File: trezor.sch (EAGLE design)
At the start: 35 parts, among them IC1 MCP1703CB, Q2 16MHz, U1 ATSHA204-TSU, U2 USB, U3 DISPLAY, X3 SSW-103-02-S-D

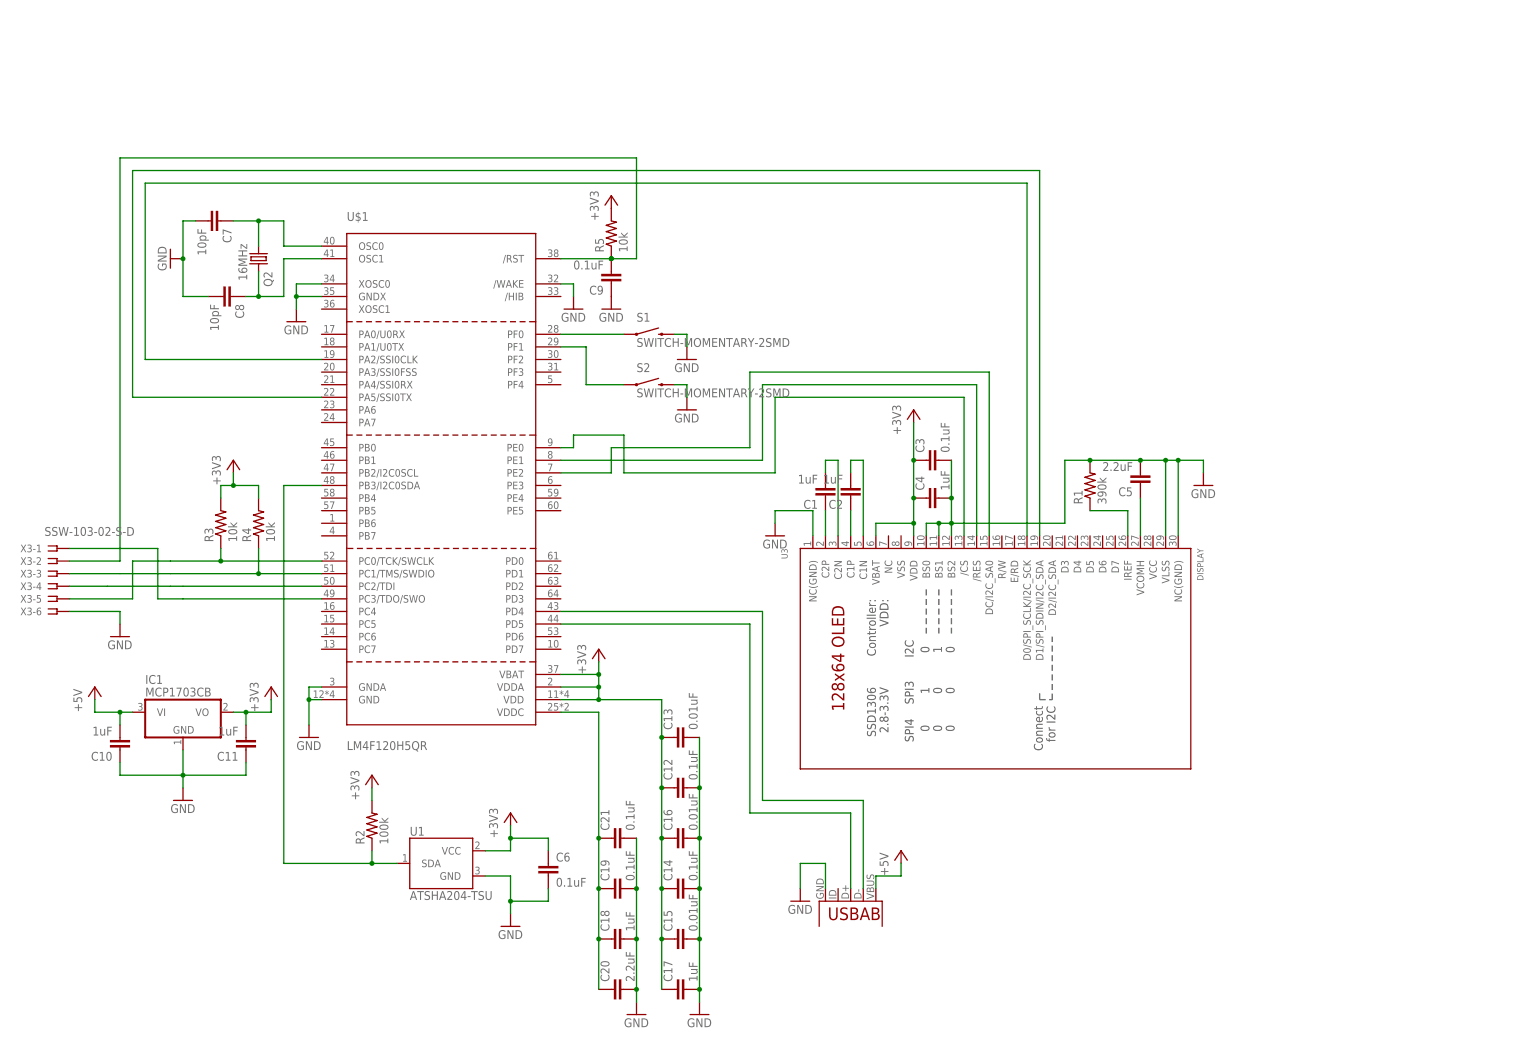
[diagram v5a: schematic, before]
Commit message: rework to STM32 (WIP)
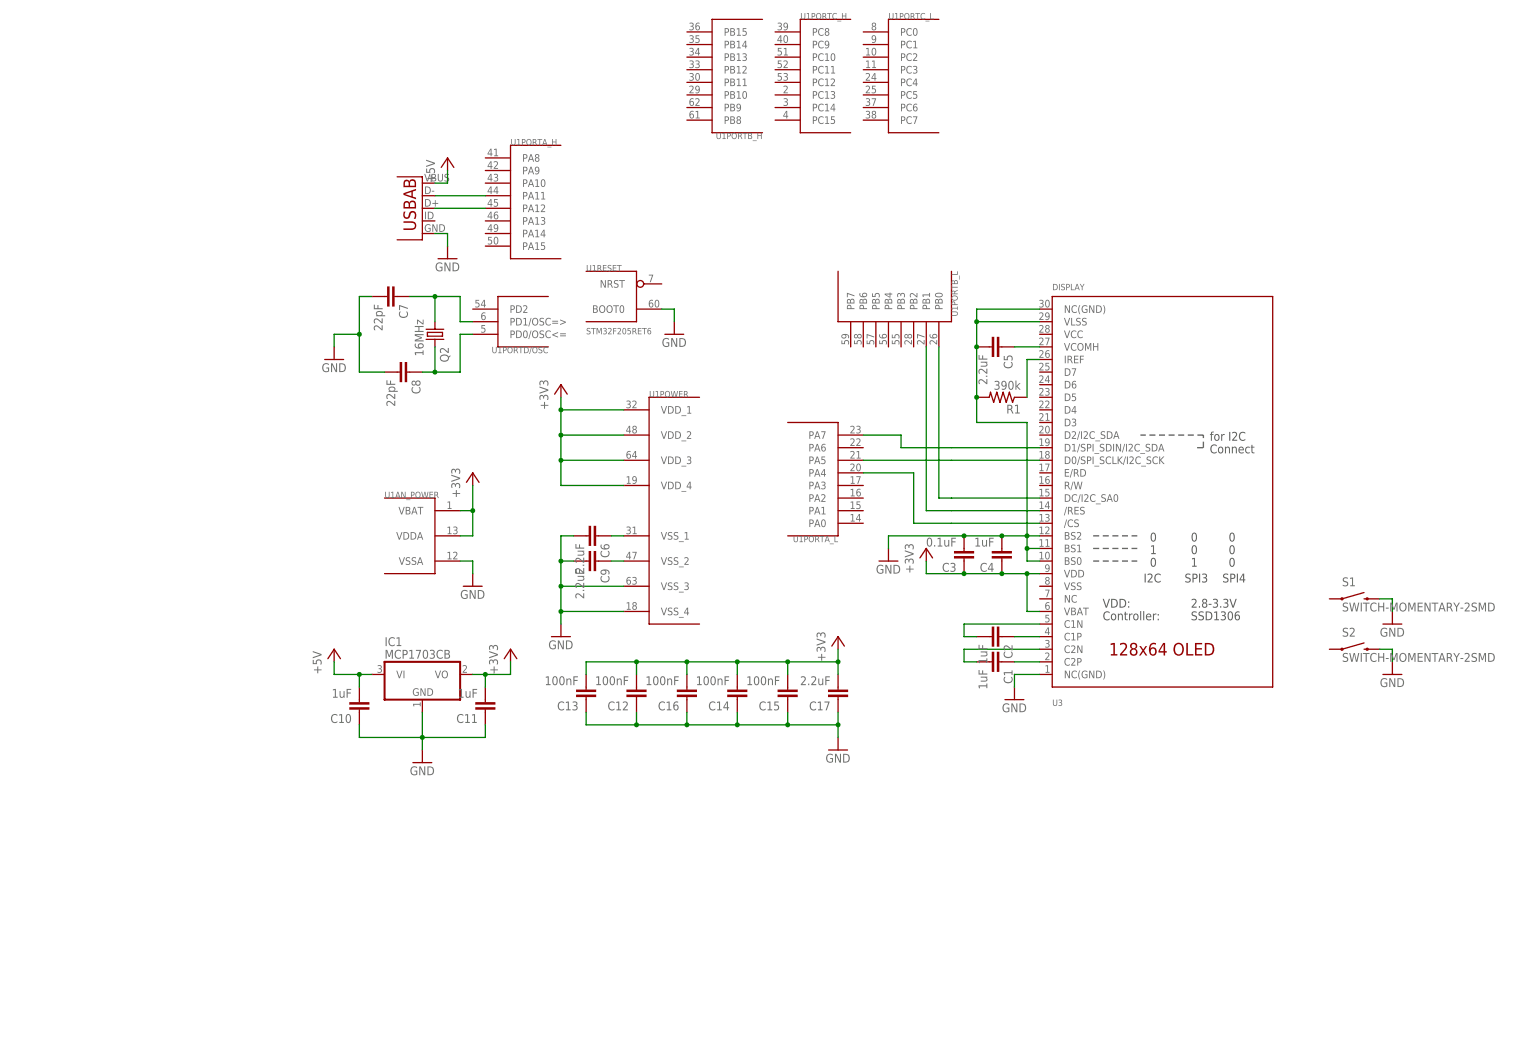
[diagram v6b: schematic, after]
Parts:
- removed C18: 1uF, SparkFun-Passives:CAP0402-CAP
- removed C19, C21: 0.1uF, SparkFun-Passives:CAP0402-CAP
- removed C20: 2.2uF, SparkFun-Passives:CAP0805
- removed R2: 100k, SparkFun-Passives:RESISTOR0402-RES
- removed R3, R4, R5: 10k, SparkFun-Passives:RESISTOR0402-RES
- removed U$1: LM4F120H5QR, stellaris:LM4F120H5QR
- removed X3: SSW-103-02-S-D, con-samtec:SSW-103-02-S-D
- C1, C10, C11, C2, C3, C4, C5: device SparkFun-Passives:CAP0402-CAP -> SparkFun-Passives:CAP0603-CAP
- C12, C14: value 0.1uF -> 100nF; device SparkFun-Passives:CAP0402-CAP -> SparkFun-Passives:CAP0603-CAP
- C13, C15, C16: value 0.01uF -> 100nF; device SparkFun-Passives:CAP0402-CAP -> SparkFun-Passives:CAP0603-CAP
- C17: value 1uF -> 2.2uF; device SparkFun-Passives:CAP0402-CAP -> SparkFun-Passives:CAP0603-CAP
- C6, C9: value 0.1uF -> 2.2uF; device SparkFun-Passives:CAP0402-CAP -> SparkFun-Passives:CAP0603-CAP
- C7, C8: value 10pF -> 22pF; device SparkFun-Passives:CAP0402-CAP -> SparkFun-Passives:CAP0603-CAP
- R1: device SparkFun-Passives:RESISTOR0402-RES -> SparkFun-Passives:RESISTOR0603-RES
- U1: value ATSHA204-TSU -> STM32F205RET6; device SparkFun-DigitalIC:ATSHA204-TSU -> stm32:STM32F10XRXT6
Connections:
- removed net N$15: S1.1, U$1.PF0
- removed net N$17: R3.1, U$1.PC0/TCK/SWCLK, X3-5.1
- removed net N$19: U$1.PC2/TDI, X3-4.1
- removed net N$20: U$1.PC3/TDO/SWO, X3-1.1
- removed net N$21: C9.2, R5.1, U$1./RST, X3-2.1
- removed net N$23: C18.1, C19.1, C20.1, C21.1, U$1.VDDC
- removed net SDA: R2.1, U$1.PB3/I2C0SDA, U1.SDA
- removed net USB_D_N: U$1.PD4, U2.D-
- removed net USB_D_P: U$1.PD5, U2.D+
- new net N$3: U1PORTB_L.PB0, U3.DC/I2C_SA0
- new net N$7: U1PORTB_L.PB1, U3./RES
- net +3V3: now also C12.2, C13.2, C14.2, C15.2, C16.2, C17.2, U1AN_POWER.VBAT, U1AN_POWER.VDDA, U1POWER.VDD_1, U1POWER.VDD_2, U1POWER.VDD_3, U1POWER.VDD_4; no longer C12.1, C13.1, C14.1, C15.1, C16.1, C17.1, C6.1, R2.2, R3.2, R4.2, R5.2, U$1.VBAT, U$1.VDD, U$1.VDDA, U1.VCC
- net GND: now also C12.1, C13.1, C14.1, C15.1, C16.1, C17.1, C9.2, U1AN_POWER.VSSA, U1POWER.VSS_3, U1POWER.VSS_4, U1RESET.BOOT0; no longer C12.2, C13.2, C14.2, C15.2, C16.2, C17.2, C18.2, C19.2, C20.2, C21.2, C9.1, U$1./WAKE, U$1.GND, U$1.GNDA, U$1.GNDX, U$1.XOSC0, U1.GND, X3-6.1
- net N$1: now also U1PORTA_L.PA7; no longer U$1.PA5/SSI0TX
- net N$14: now also U1PORTA_H.PA12, U2.D+; no longer S2.1, U$1.PF1
- net N$16: now also U1PORTA_L.PA4, U3./CS; no longer R4.1, U$1.PC1/TMS/SWDIO, X3-3.1
- net N$2: now also U1PORTA_H.PA11, U2.D-; no longer U$1.PE0, U3./CS
- net N$4: now also C6.1, U1POWER.VSS_1; no longer U$1.PE2, U3.DC/I2C_SA0
- net N$5: now also U1PORTA_L.PA5; no longer U$1.PA2/SSI0CLK
- net N$8: now also C9.1, U1POWER.VSS_2; no longer U$1.PE1, U3./RES
- net XTAL1: now also U1PORTD/OSC.PD1/OSC=>; no longer U$1.OSC0
- net XTAL2: now also U1PORTD/OSC.PD0/OSC<=; no longer U$1.OSC1
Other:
- moved on the sheet: C1, C10, C11, C12, C13, C14, C15, C16, C17, C2, C3, C4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
